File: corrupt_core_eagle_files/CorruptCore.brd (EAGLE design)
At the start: 100 x 58 mm, 91 parts, among them K1 DTS-3, K10 DTS-3, K11 DTS-3, K12 DTS-3, K13 DTS-3, K14 DTS-3, K15 DTS-3, K16 DTS-3, K2 DTS-3, K3 DTS-3, K4 DTS-3, K5 DTS-3, K6 DTS-3, K7 DTS-3, K8 DTS-3, K9 DTS-3, U1 MEGA8-P, U2 SNX4HC595SOIC16, U3 SNX4HC595SOIC16, U4 SNX4HC595SOIC16, U5 ULN2803ASOIC18, U6 ULN2803ASOIC18, U7 ULN2803ASOIC18, U8 LTC1799, Y1 16MHz

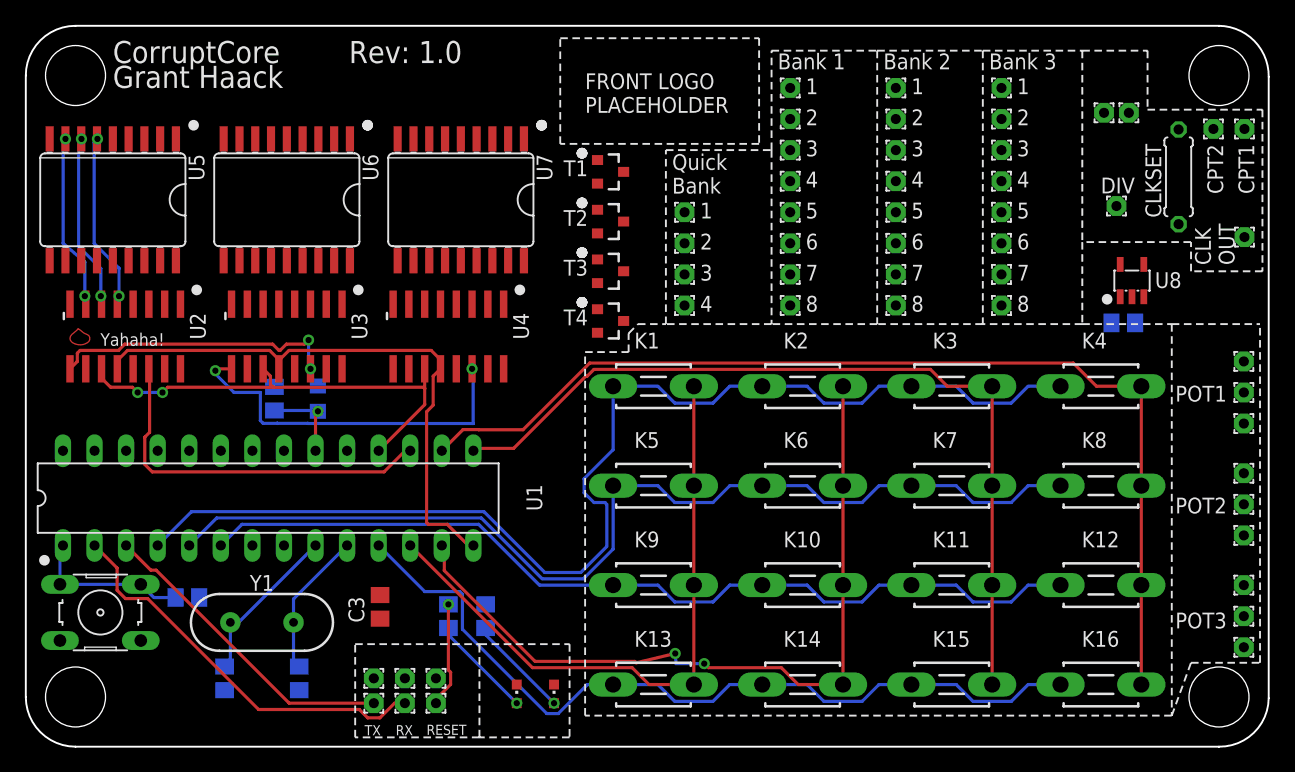
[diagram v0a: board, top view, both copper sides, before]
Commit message: apparently I never pushed this
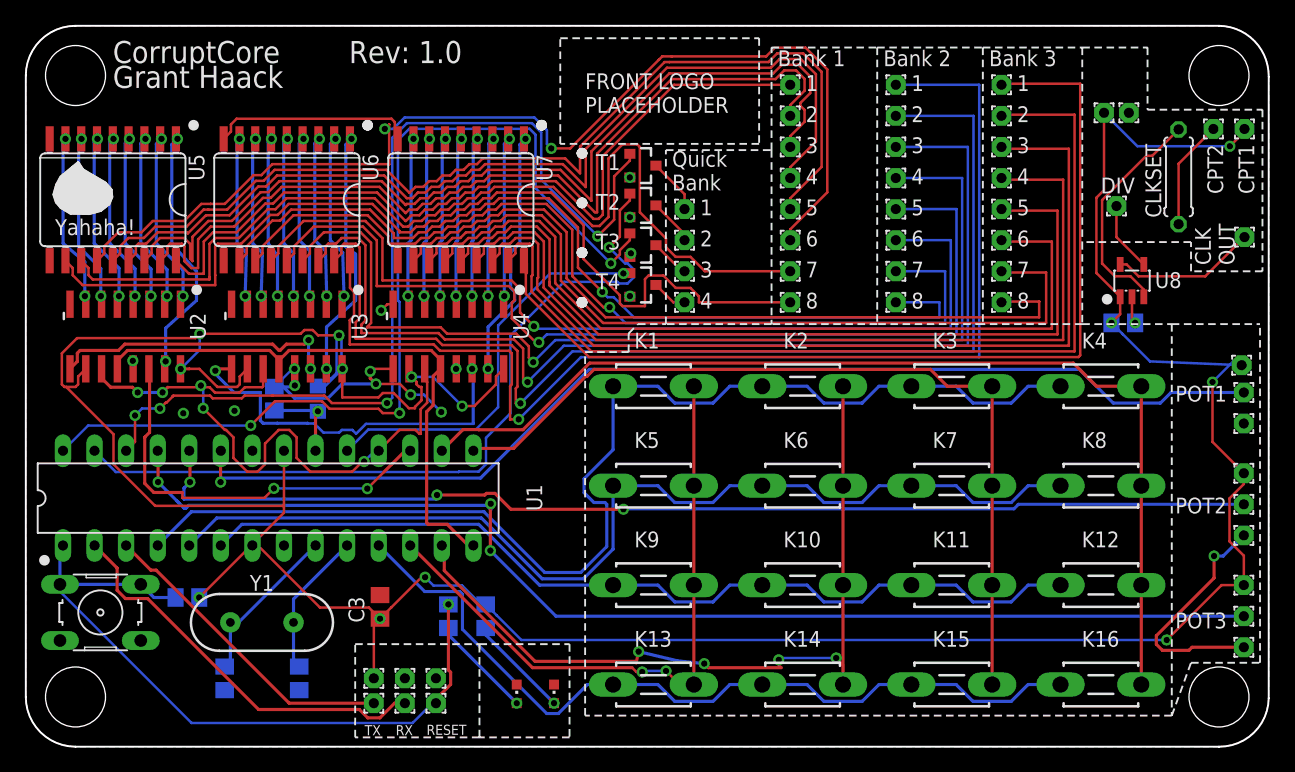
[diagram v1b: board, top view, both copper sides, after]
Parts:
- moved T4 3.89 mm to (49.6, 37.1)
- moved T3 3.34 mm to (49.6, 40.4)
- moved T2 2.91 mm to (49.6, 43.5)
- moved T1 2.65 mm to (49.6, 46.8)
- moved 5V@POT1 0.35 mm to (97.8, 30.7)
- moved B1_P1 0.25 mm to (61.5, 53.3)
- moved B1_P2 0.25 mm to (61.5, 50.8)
- moved B1_P3 0.25 mm to (61.5, 48.3)
- moved B1_P4 0.25 mm to (61.5, 45.8)
- moved B1_P5 0.25 mm to (61.5, 43.3)
- moved B1_P6 0.25 mm to (61.5, 40.8)
- moved B1_P7 0.25 mm to (61.5, 38.3)
- moved B1_P8 0.25 mm to (61.5, 35.8)
- moved B2_P1 0.25 mm to (70.0, 53.3)
- moved B2_P2 0.25 mm to (70.0, 50.8)
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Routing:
- net +5V: track 0.00 -> 267.4 mm, vias 0 -> 13
- net POT3: track 0.00 -> 97.8 mm, vias 0 -> 3
- net B2_P1: track 0.00 -> 94.2 mm, vias 0 -> 1
- net B2_P2: track 0.00 -> 92.0 mm, vias 0 -> 1
- net POT2: track 0.00 -> 90.4 mm, vias 0 -> 3
- net POT1: track 0.00 -> 90.3 mm, vias 0 -> 1
- net B1_P6: track 0.00 -> 87.5 mm, vias 0 -> 2
- net B2_P3: track 0.00 -> 87.3 mm, vias 0 -> 1
- net B2_P4: track 0.00 -> 82.8 mm, vias 0 -> 1
- net B1_P5: track 0.00 -> 80.7 mm
- net B1_P7: track 0.00 -> 79.2 mm
- net QP3: track 0.00 -> 78.7 mm, vias 0 -> 3
- net B2_P5: track 0.00 -> 78.2 mm, vias 0 -> 1
- net B3_P1: track 0.00 -> 77.8 mm
- net B3_P2: track 0.00 -> 77.3 mm
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- added copper zone on layer 1, net GND
- added copper zone on layer 16, net GND
- removed copper zone on layer 1, net N$15
